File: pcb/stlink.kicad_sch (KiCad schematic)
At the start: 37 parts, among them J1 USB_A, Q1 S9013, U1 XC6206P332MR, U2 STM32F103CB, Y1 8MHz

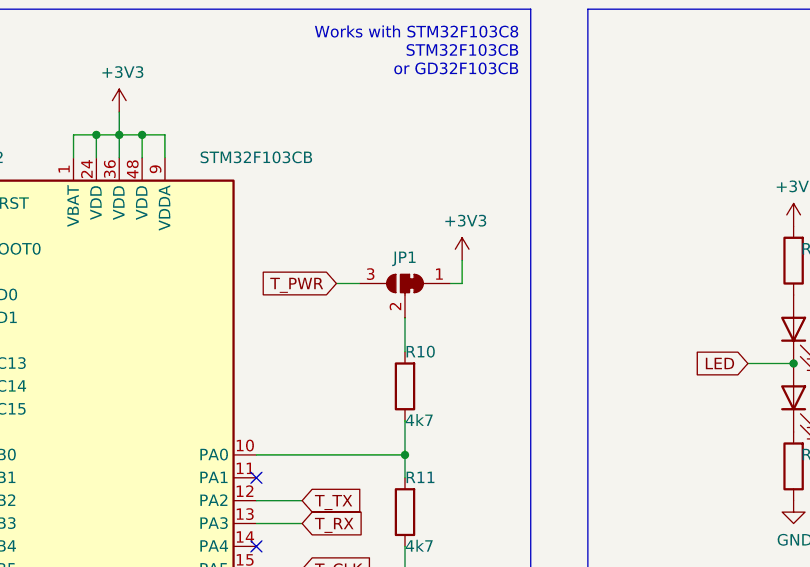
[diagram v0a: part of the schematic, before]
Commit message: Hmmmm
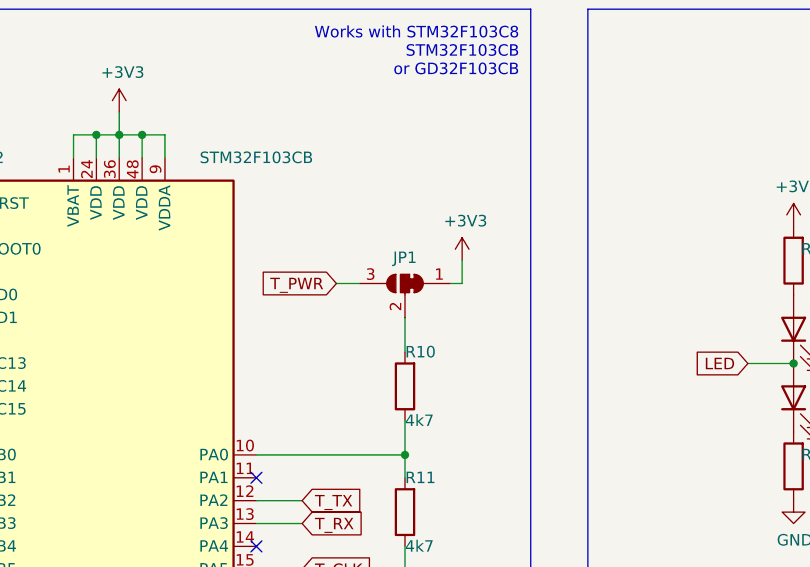
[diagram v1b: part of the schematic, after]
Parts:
- J1: LCSC (none) -> C112454
